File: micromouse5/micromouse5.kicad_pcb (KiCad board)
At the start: 2 copper layers, 75 x 105 mm, 71 parts, among them J1 Conn_01x06_Pin, J2 Conn_01x06_Pin, J3 JST 2, J4 JST 1, J5 Conn_01x04_Pin, Q1 IR Receiver, Q2 IR Receiver, Q3 IR Receiver, Q4 IR Receiver, SW1 Button, SW2 EG1218, U1 HBridge, U2 Voltage Regulator, U3 MOSFET, U4 MOSFET, U5 MOSFET, U6 MOSFET, U7 STM32F205RGTx

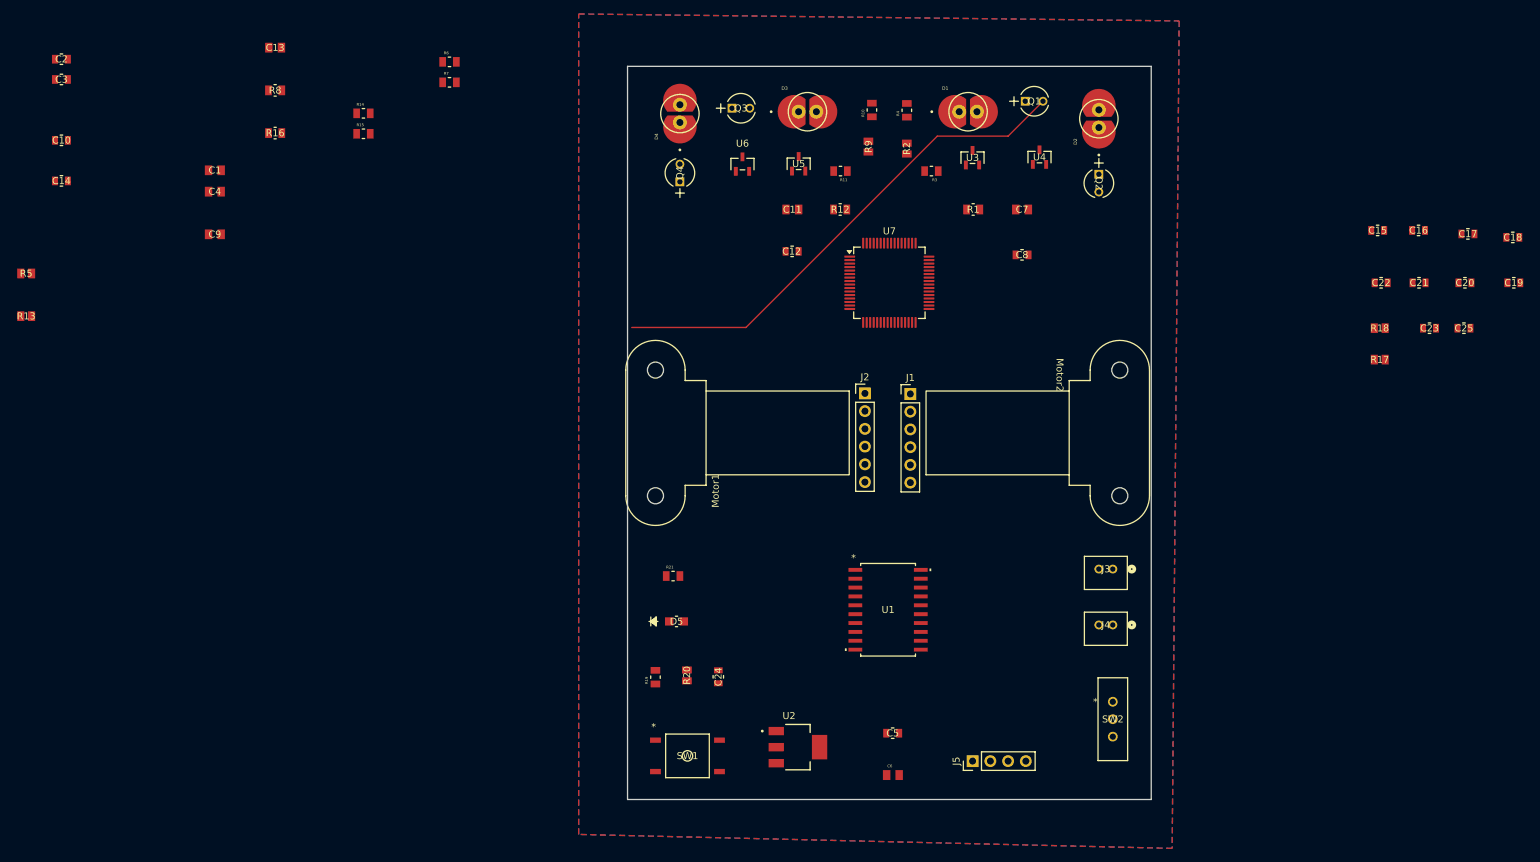
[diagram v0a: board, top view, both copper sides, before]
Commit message: pcb work
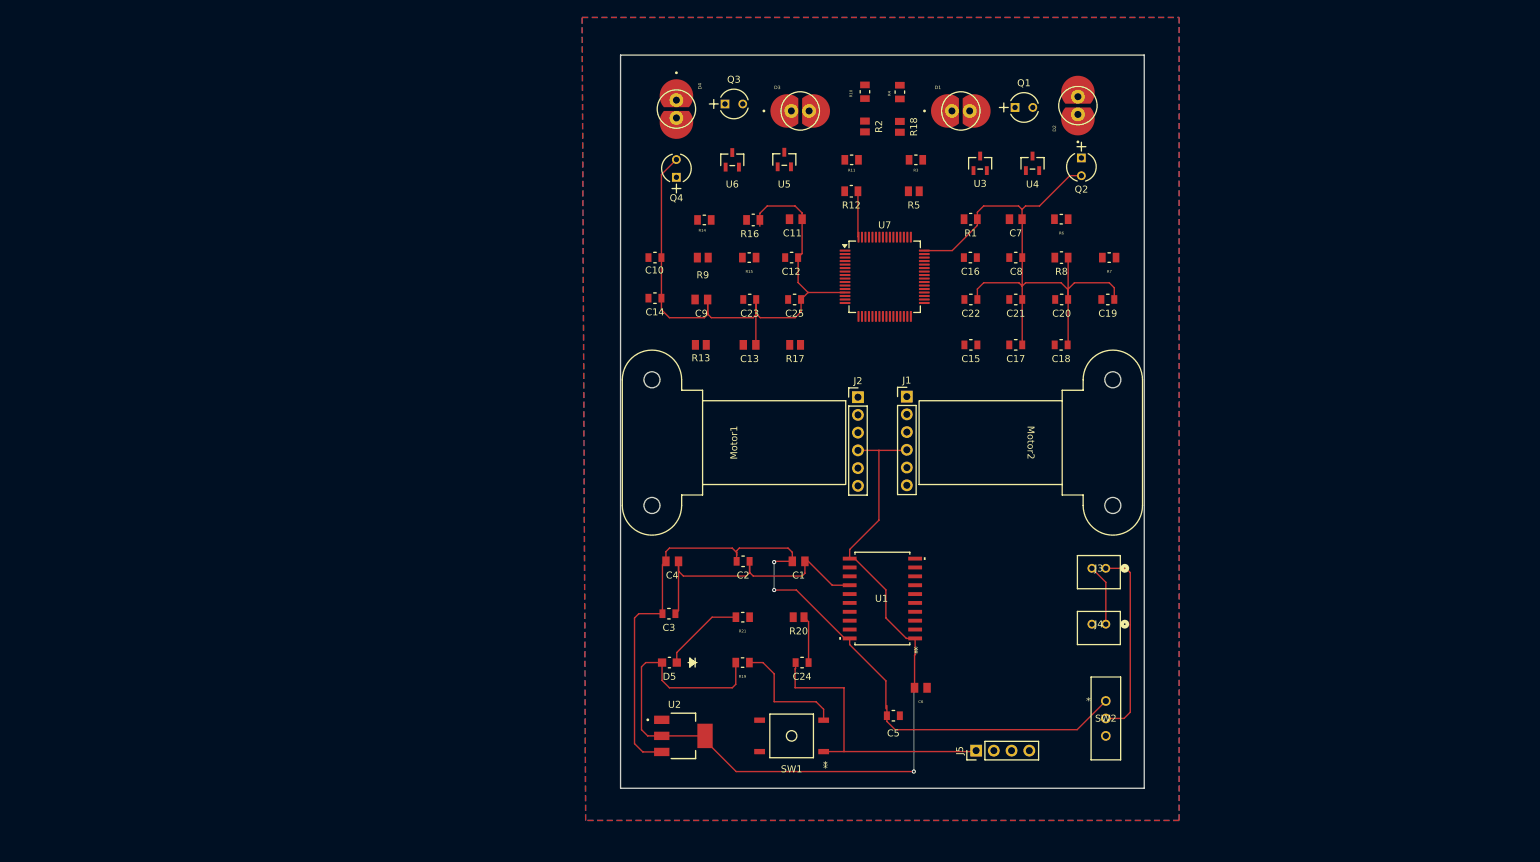
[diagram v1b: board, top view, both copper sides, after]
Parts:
- moved R5 127.7 mm to (177.0, 69.9)
- moved C2 121.3 mm to (152.6, 122.9)
- moved C3 115.9 mm to (141.9, 130.4), turned to 180 degrees
- moved R8 115.1 mm to (198.1, 79.4)
- moved C1 100.6 mm to (160.5, 122.9), turned to 180 degrees
- moved R7 97.8 mm to (205.0, 79.4)
- moved C23 97.4 mm to (153.5, 85.4), turned to 180 degrees
- moved R13 96.7 mm to (146.5, 91.9)
- moved C25 95.9 mm to (159.9, 85.4), turned to 180 degrees
- moved R6 90.5 mm to (198.1, 73.9)
- moved C10 86.6 mm to (139.9, 79.4)
- moved C14 86.6 mm to (139.9, 85.2)
- moved C4 84.2 mm to (142.4, 122.9)
- moved R17 83.8 mm to (160.0, 91.9), turned to 180 degrees
- moved C13 80.2 mm to (153.5, 91.9)
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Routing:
- net 3V3: track 72.3 -> 310.9 mm, vias 0 -> 1
- net VCC: track 0.00 -> 126.3 mm, vias 0 -> 2
- net NRST: track 0.00 -> 41.7 mm
- net MGND: track 0.00 -> 40.8 mm
- net Net-(J3-Pad1): track 0.00 -> 27.6 mm
- net Net-(R19-Pad2): track 0.00 -> 17.3 mm
- net Net-(D5-K): track 0.00 -> 12.0 mm
- net Net-(J3-Pad2): track 0.00 -> 8.83 mm
- net Net-(C24-Pad2): track 0.00 -> 6.77 mm
